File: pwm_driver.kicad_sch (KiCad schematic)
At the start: 12 parts, among them J3 Conn_01x16_Pin, J4 Conn_01x16_Pin, J5 Conn_01x16_Pin, J6 Conn_01x16_Pin, J7 Conn_01x16_Pin, J8 Conn_01x16_Pin, U5 PCA9685PW, U6 PCA9685PW

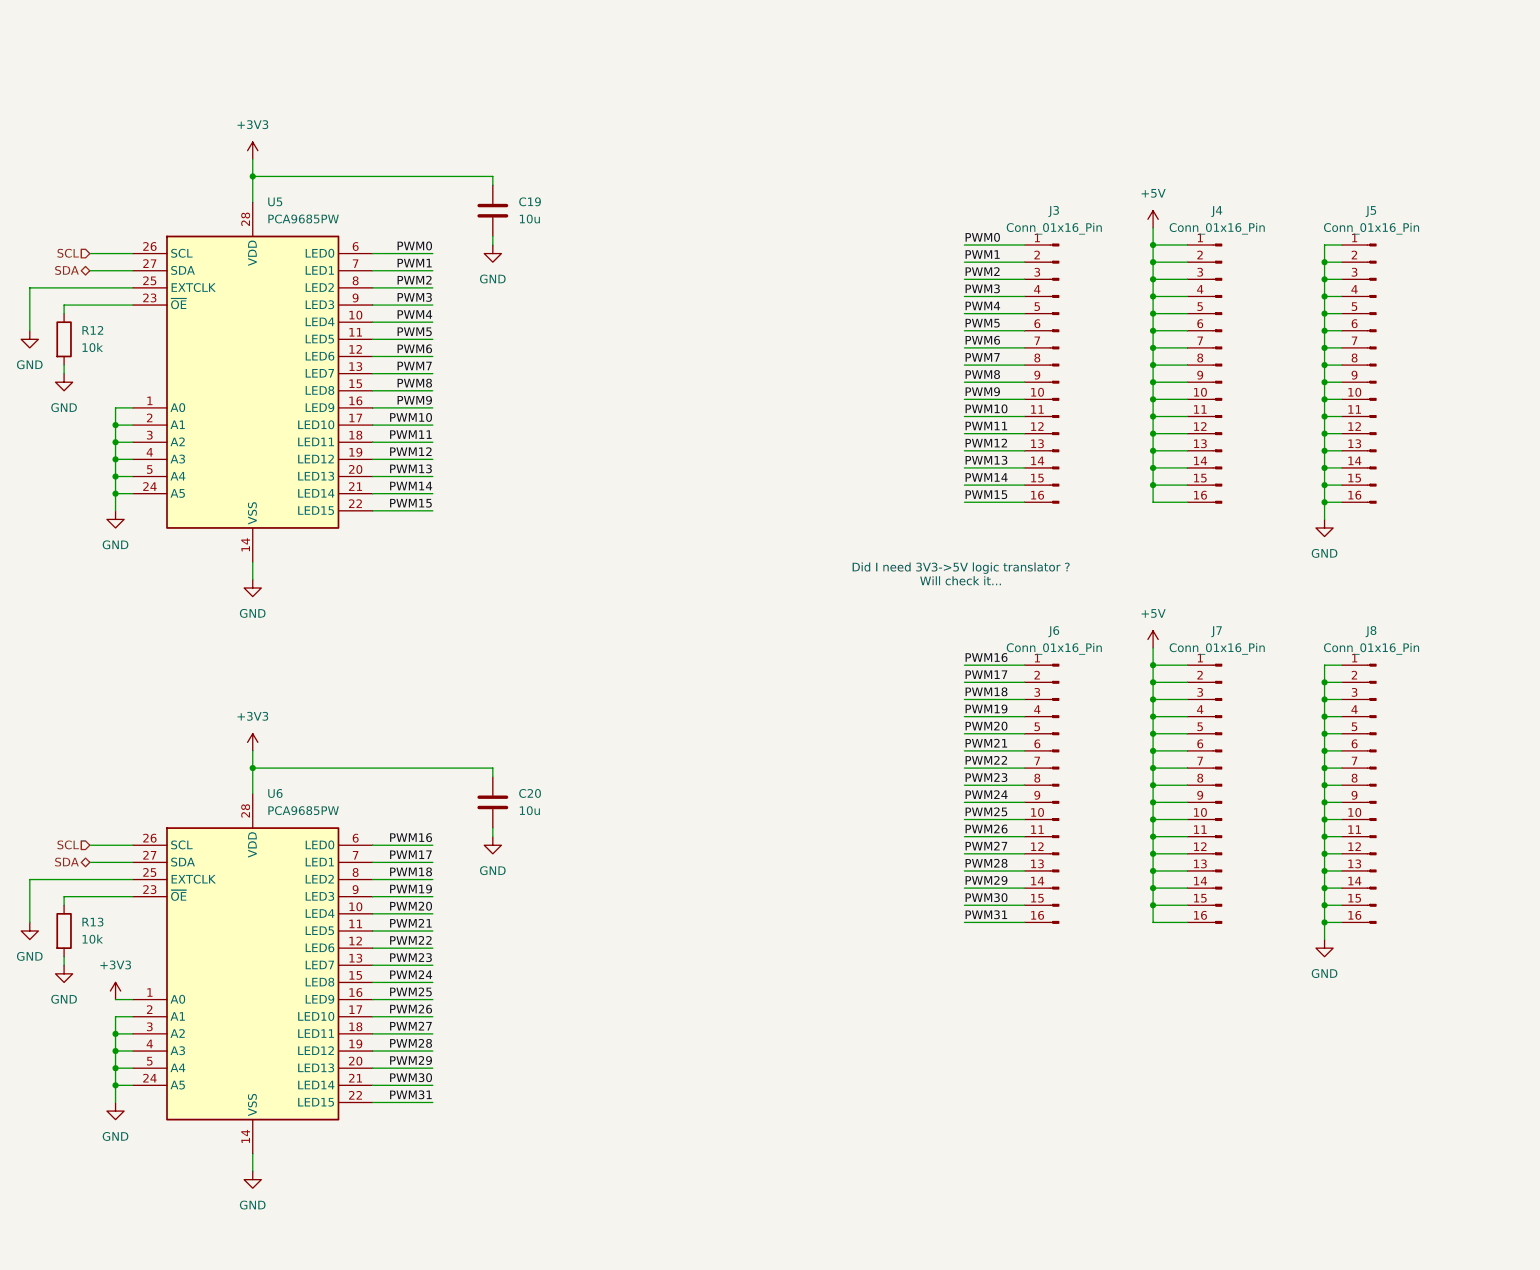
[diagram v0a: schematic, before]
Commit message: Update schematic
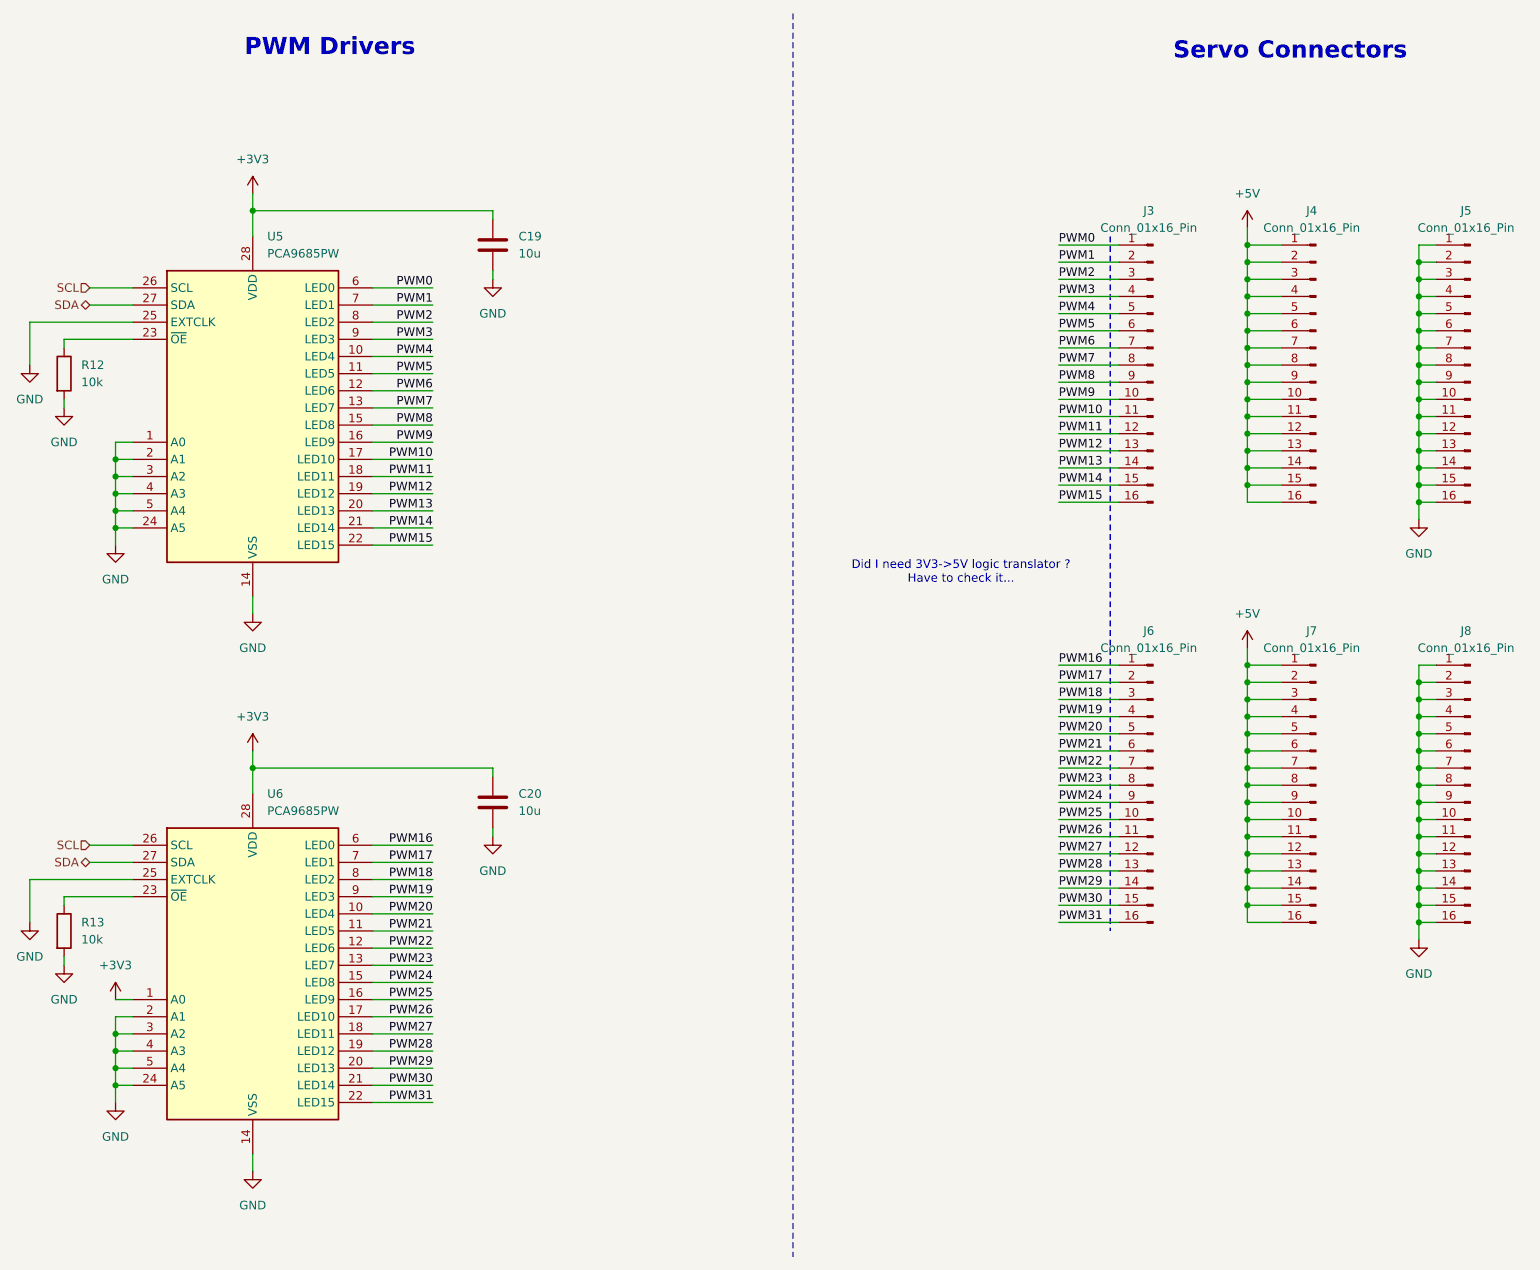
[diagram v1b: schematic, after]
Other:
- note added: "Did I need 3V3->5V logic translator ? Have to check it..."
- note added: "PWM Drivers"
- note added: "Servo Connectors"
- note removed: "Did I need 3V3->5V logic translator ? Will check it..."
- moved on the sheet: C19, J3, J4, J5, J6, J7, J8, R12, U5
